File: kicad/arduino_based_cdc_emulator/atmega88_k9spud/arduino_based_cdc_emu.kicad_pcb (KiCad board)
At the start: 2 copper layers, 13 parts, among them IC1 ATMEGA88-A, P1 CONN_5, P2 CONN_2, U1 78L05, X1 20MHz

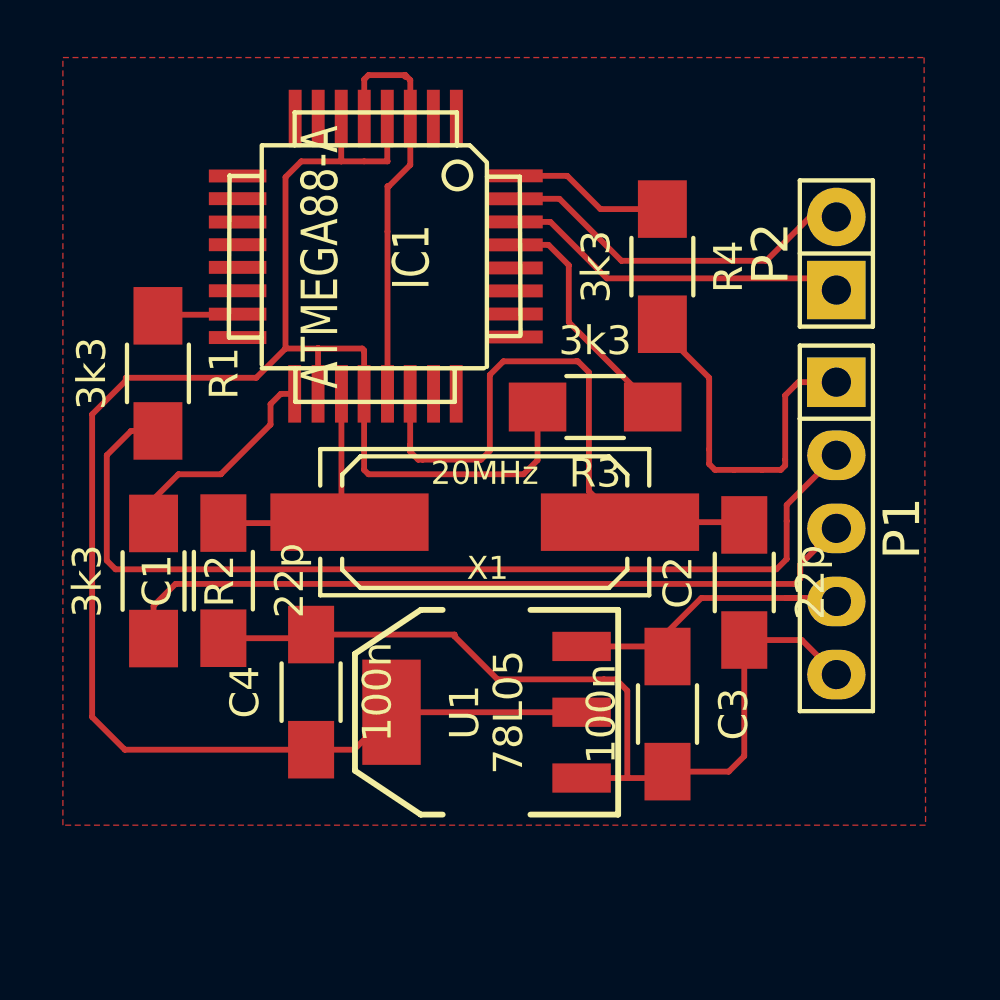
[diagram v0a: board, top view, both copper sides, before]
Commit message: updates
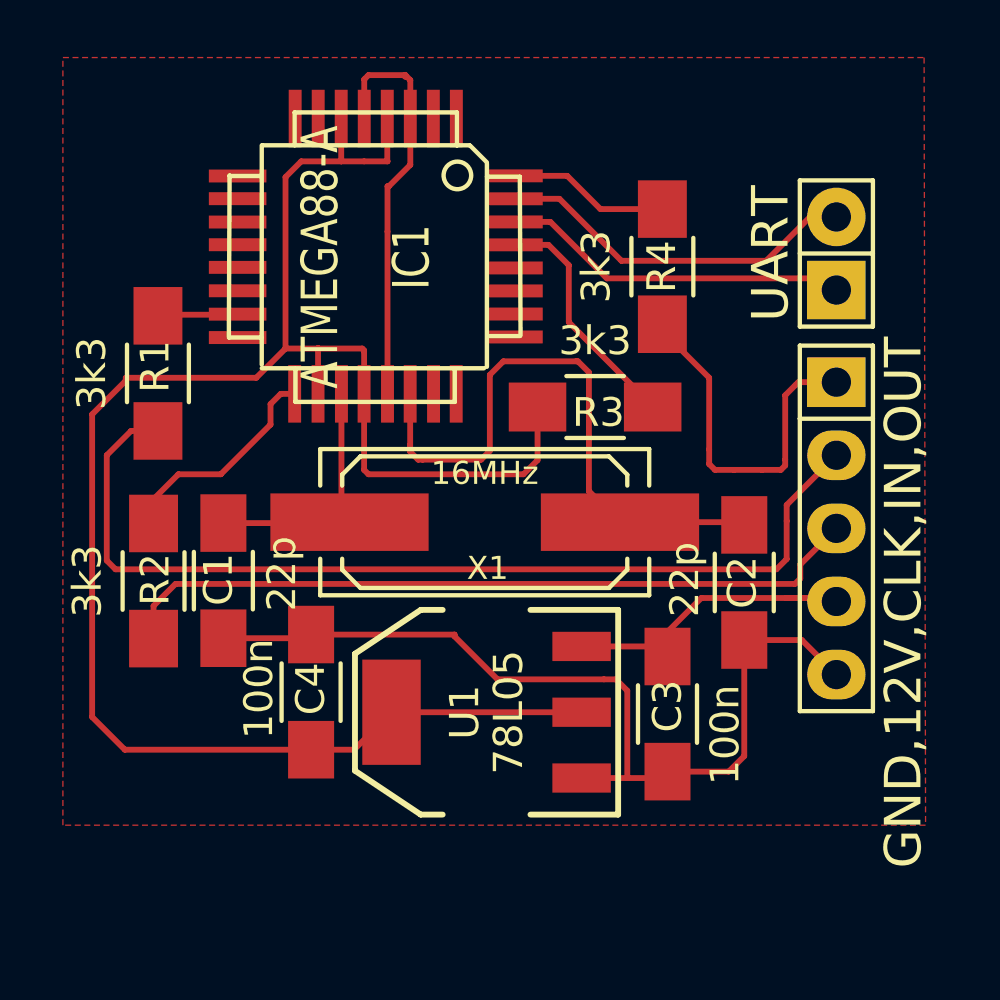
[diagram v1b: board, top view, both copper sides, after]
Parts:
- X1: value 20MHz -> 16MHz
- renumbered P1 to GND,12V,CLK,IN,OUT, P2 to UART
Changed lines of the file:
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@@
-(kicad_pcb (version 4) (host pcbnew "(2014-jul-16 BZR unknown)-product")
+(kicad_pcb (version 20170123) (host pcbnew no-vcs-found-7602~57~ubuntu16.04.1)
   (general
     (links 30)
     (no_connects 0)
-    (area 113.158657 102.6668 144.943286 129.336801)
+    (area 113.8333 102.6668 144.597 131.420124)
     (thickness 1.6002)
     (drawings 0)
@@
   )
   (layers
-    (0 Front signal)
-    (31 Back signal)
-    (32 B.Adhes user)
-    (33 F.Adhes user)
-    (34 B.Paste user)
-    (35 F.Paste user)
-    (36 B.SilkS user)
+    (0 Front signal hide)
+    (31 Back signal hide)
+    (32 B.Adhes user hide)
+    (33 F.Adhes user hide)
+    (34 B.Paste user hide)
+    (35 F.Paste user hide)
+    (36 B.SilkS user hide)
     (37 F.SilkS user)
-    (38 B.Mask user)
-    (39 F.Mask user)
-    (40 Dwgs.User user)
-    (41 Cmts.User user)
-    (42 Eco1.User user)
-    (43 Eco2.User user)
-    (44 Edge.Cuts user)
+    (38 B.Mask user hide)
+    (39 F.Mask user hide)
+    (40 Dwgs.User user hide)
+    (41 Cmts.User user hide)
+    (42 Eco1.User user hide)
+    (43 Eco2.User user hide)
+    (44 Edge.Cuts user hide)
   )
   (setup
@@
     (pad_to_mask_clearance 0.254)
     (aux_axis_origin 0 0)
-    (visible_elements FFFFFF7F)
+    (visible_elements FFFFFD7F)
     (pcbplotparams
-      (layerselection 0x00030_80000001)
+      (layerselection 0x00020_7fffffff)
       (usegerberextensions true)
       (excludeedgelayer true)
@@
       (hpglpenspeed 20)
       (hpglpendiameter 15)
-      (hpglpenoverlay 2)
       (psnegative false)
       (psa4output false)
@@
       (outputformat 1)
       (mirror false)
-      (drillshape 1)
+      (drillshape 0)
       (scaleselection 1)
-      (outputdirectory ""))
+      (outputdirectory /home/nail/tmp/plot/))
   )
   (net 0 "")
@@
     (tags "capacitor 1206")
     (attr smd)
-    (fp_text reference C1 (at 0 -2.3 90) (layer F.SilkS)
-      (effects (font (size 1 1) (thickness 0.15)))
-    )
-    (fp_text value 22p (at 0 2.3 90) (layer F.SilkS)
+    (fp_text reference C1 (at 0.0405 -0.1705 90) (layer F.SilkS)
+      (effects (font (size 1 1) (thickness 0.15)))
+    )
+    (fp_text value 22p (at 0.2405 2.0295 90) (layer F.SilkS)
       (effects (font (size 1 1) (thickness 0.15)))
     )
@@
     (tags "capacitor 1206")
     (attr smd)
-    (fp_text reference C2 (at 0 -2.3 90) (layer F.SilkS)
-      (effects (font (size 1 1) (thickness 0.15)))
-    )
-    (fp_text value 22p (at 0 2.3 90) (layer F.SilkS)
+    (fp_text reference C2 (at 0 -0.068 90) (layer F.SilkS)
+      (effects (font (size 1 1) (thickness 0.15)))
+    )
+    (fp_text value 22p (at 0.104 -2.068 90) (layer F.SilkS)
       (effects (font (size 1 1) (thickness 0.15)))
     )
@@
     (tags "capacitor 1206")
     (attr smd)
-    (fp_text reference C3 (at 0 -2.3 270) (layer F.SilkS)
-      (effects (font (size 1 1) (thickness 0.15)))
-    )
-    (fp_text value 100n (at 0 2.3 270) (layer F.SilkS)
+    (fp_text reference C3 (at -0.276 0.001 270) (layer F.SilkS)
+      (effects (font (size 1 1) (thickness 0.15)))
+    )
+    (fp_text value 100n (at 0.724 -1.999 270) (layer F.SilkS)
       (effects (font (size 1 1) (thickness 0.15)))
     )
@@
     (tags "capacitor 1206")
     (attr smd)
-    (fp_text reference C4 (at 0 -2.3 90) (layer F.SilkS)
-      (effects (font (size 1 1) (thickness 0.15)))
-    )
-    (fp_text value 100n (at 0 2.3 90) (layer F.SilkS)
+    (fp_text reference C4 (at 0.114 -0.0185 90) (layer F.SilkS)
+      (effects (font (size 1 1) (thickness 0.15)))
+    )
+    (fp_text value 100n (at 0.114 -1.8185 90) (layer F.SilkS)
       (effects (font (size 1 1) (thickness 0.15)))
     )
@@
     (descr "Through hole pin header")
     (tags "pin header")
-    (fp_text reference P1 (at 0 -2.286 270) (layer F.SilkS)
+    (fp_text reference GND,12V,CLK,IN,OUT (at 2.5756 -2.3316 270) (layer F.SilkS)
       (effects (font (size 1.27 1.27) (thickness 0.2032)))
     )
@@
     (tags "resistor 1206")
     (attr smd)
-    (fp_text reference R1 (at 0 -2.3 270) (layer F.SilkS)
+    (fp_text reference R1 (at -0.2396 0.0972 270) (layer F.SilkS)
       (effects (font (size 1 1) (thickness 0.15)))
     )
@@
     (tags "resistor 1206")
     (attr smd)
-    (fp_text reference R2 (at 0 -2.3 270) (layer F.SilkS)
+    (fp_text reference R2 (at -0.0532 -0.0552 270) (layer F.SilkS)
       (effects (font (size 1 1) (thickness 0.15)))
     )
@@
     (tags "resistor 1206")
     (attr smd)
-    (fp_text reference R3 (at 0 -2.3 180) (layer F.SilkS)
+    (fp_text reference R3 (at -0.1136 -0.192 180) (layer F.SilkS)
       (effects (font (size 1 1) (thickness 0.15)))
     )
@@
     (tags "resistor 1206")
     (attr smd)
-    (fp_text reference R4 (at 0 -2.3 270) (layer F.SilkS)
+    (fp_text reference R4 (at 0 0.0232 270) (layer F.SilkS)
       (effects (font (size 1 1) (thickness 0.15)))
     )
@@
       (effects (font (size 0.8 0.8) (thickness 0.15)))
     )
-    (fp_text value 20MHz (at 0 1.7 180) (layer F.SilkS)
+    (fp_text value 16MHz (at 0 1.7 180) (layer F.SilkS)
       (effects (font (size 0.8 0.8) (thickness 0.15)))
     )
@@
     (descr "Through hole pin header")
     (tags "pin header")
-    (fp_text reference P2 (at 0 -2.286 90) (layer F.SilkS)
+    (fp_text reference UART (at 0 -2.286 90) (layer F.SilkS)
       (effects (font (size 1.27 1.27) (thickness 0.2032)))
     )
